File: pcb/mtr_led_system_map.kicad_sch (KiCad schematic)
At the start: 489 parts, among them J1 USB_C_Receptacle_USB2.0_16P, U1 ESP32-S3-WROOM-1, U2 AP2112K-3.3

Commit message: Updated the schematic to use dual red/yellow LEDs
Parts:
- removed DR_DOOR_1, DY_ISL_ADM1, DY_ISL_CAB1, DY_ISL_CEN1, DY_ISL_CHW1, DY_ISL_FOH1, DY_ISL_HAH1, DY_ISL_HFC1, DY_ISL_HKU1, DY_ISL_KET1, DY_ISL_NOP1, DY_ISL_POA1, DY_ISL_QUB1, DY_ISL_SHW1, DY_ISL_SKW1, DY_ISL_SWH1, DY_ISL_SYP1, DY_ISL_TAK1, DY_ISL_TIH1, DY_ISL_WAC1, DY_KTL_CHH1, DY_KTL_DIH1, DY_KTL_HOM1, DY_KTL_KOB1, DY_KTL_KOT1, DY_KTL_KWT1, DY_KTL_LAT1, DY_KTL_LOF1, DY_KTL_MOK1, DY_KTL_NTK1, DY_KTL_PRE1, DY_KTL_SKM1, DY_KTL_TIK1, DY_KTL_WHA1, DY_KTL_WTS1, DY_KTL_YAT1, DY_KTL_YMT1, DY_TKL_LHP1, DY_TKL_NOP1, DY_TKL_QUB1, DY_TKL_TIK1, DY_TKL_TKO1, DY_TKL_YAT1, DY_TWL_ADM1, DY_TWL_CEN1, DY_TWL_CSW1, DY_TWL_JOR1, DY_TWL_KWF1, DY_TWL_KWH1, DY_TWL_LAK1, DY_TWL_LCK1, DY_TWL_MEF1, DY_TWL_MOK1, DY_TWL_PRE1, DY_TWL_SSP1, DY_TWL_TST1, DY_TWL_TSW1, DY_TWL_TWH1, DY_TWL_YMT1: YELLOW, LED_SMD:LED_0805_2012Metric, symbol Device:LED
- removed DR_DOOR_2: GREEN, LED_SMD:LED_0805_2012Metric, symbol Device:LED
- removed DR_ISL_ADM1, DR_ISL_CAB1, DR_ISL_CEN1, DR_ISL_CHW1, DR_ISL_FOH1, DR_ISL_HFC1, DR_ISL_HKU1, DR_ISL_KET1, DR_ISL_NOP1, DR_ISL_QUB1, DR_ISL_SHW1, DR_ISL_SKW1, DR_ISL_SWH1, DR_ISL_SYP1, DR_ISL_TAK1, DR_ISL_TIH1, DR_ISL_WAC1, DR_KTL_CHH1, DR_KTL_DIH1, DR_KTL_HOM1, DR_KTL_KOB1, DR_KTL_KOT1, DR_KTL_KWT1, DR_KTL_LAT1, DR_KTL_LOF1, DR_KTL_MOK1, DR_KTL_NTK1, DR_KTL_PRE1, DR_KTL_SKM1, DR_KTL_TIK1, DR_KTL_WHA1, DR_KTL_WTS1, DR_KTL_YAT1, DR_KTL_YMT1, DR_TKL_HAH1, DR_TKL_LHP1, DR_TKL_NOP1, DR_TKL_POA1, DR_TKL_QUB1, DR_TKL_TIK1, DR_TKL_TKO1, DR_TKL_YAT1, DR_TWL_ADM1, DR_TWL_CEN1, DR_TWL_CSW1, DR_TWL_JOR1, DR_TWL_KWF1, DR_TWL_KWH1, DR_TWL_LAK1, DR_TWL_LCK1, DR_TWL_MEF1, DR_TWL_MOK1, DR_TWL_PRE1, DR_TWL_SSP1, DR_TWL_TST1, DR_TWL_TSW1, DR_TWL_TWH1, DR_TWL_YMT1: RED, LED_SMD:LED_0805_2012Metric, symbol Device:LED
- removed R1, R109, R110, R111, R112, R113, R114, R115, R116, R133, R134, R135, R136, R137, R138, R139, R140, R155, R156, R157, R158, R159, R160, R169, R170, R171, R172, R181, R182, R183, R184, R185, R186, R187, R188, R189, R190, R191, R192, R193, R194, R195, R196, R197, R198, R199, R2, R200, R201, R202, R203, R204, R205, R206, R207, R208, R209, R210, R211, R212, R213, R214, R215, R216, R217, R218, R219, R220, R221, R222, R223, R224, R225, R226, R227, R228, R229, R230, R231, R232, R233, R234, R235, R236, R237, R238, R27, R28, R29, R3, R30, R31, R32, R33, R34, R4, R5, R53, R54, R55, R56, R57, R58, R59, R6, R60, R7, R8, R83, R84, R85, R86, R87, R88, R89, R90: 220R, Resistor_SMD:R_0603_1608Metric, symbol Device:R
- added D_DOOR_G1: GREEN, LED_SMD:LED_0805_2012Metric, symbol Device:LED
- added D_DOOR_Y1: YELLOW, LED_SMD:LED_0805_2012Metric, symbol Device:LED
- added D_ISL_ADM1, D_ISL_CEN1, D_ISL_CHW1, D_ISL_CWB1, D_ISL_FOH1, D_ISL_HFC1, D_ISL_HKU1, D_ISL_KET1, D_ISL_NOP1, D_ISL_QUB1, D_ISL_SHW1, D_ISL_SKW1, D_ISL_SWH1, D_ISL_SYP1, D_ISL_TAK1, D_ISL_TIH1, D_ISL_WAC1, D_KTL_CHH1, D_KTL_DIH1, D_KTL_HOM1, D_KTL_KOB1, D_KTL_KOT1, D_KTL_KWT1, D_KTL_LAT1, D_KTL_LOF1, D_KTL_MOK1, D_KTL_NTK1, D_KTL_PRE1, D_KTL_SKM1, D_KTL_TIK1, D_KTL_WHA1, D_KTL_WTS1, D_KTL_YAT1, D_KTL_YMT1, D_TKL_HAH1, D_TKL_LHP1, D_TKL_NOP1, D_TKL_POA1, D_TKL_QUB1, D_TKL_TIK1, D_TKL_TKO1, D_TKL_YAT1, D_TWL_ADM1, D_TWL_CEN1, D_TWL_CSW1, D_TWL_JOR1, D_TWL_KWF1, D_TWL_KWH1, D_TWL_LAK1, D_TWL_LCK1, D_TWL_MEF1, D_TWL_MOK1, D_TWL_PRE1, D_TWL_SSP1, D_TWL_TST1, D_TWL_TSW1, D_TWL_TWH1, D_TWL_YMT1: RED_YELLOW, LED_SMD:LED_Kingbright_APHBM2012_2x1.25mm, symbol Device:LED_Dual_AKKA
- added R647, R648, R649, R650, R667, R668, R669, R670, R671, R672, R673, R674, R675, R676, R677, R678, R695, R696, R697, R698, R699, R700, R701, R702, R703, R704, R705, R706, R707, R708, R709, R710, R727, R728, R729, R730, R731, R732, R733, R734, R735, R736, R737, R738, R739, R740, R741, R742, R759, R760, R761, R762, R763, R764, R765, R766, R767, R768, R769, R770, R771, R772, R773, R774, R791, R792, R793, R794, R795, R796, R797, R798, R799, R800, R801, R802, R803, R804, R805, R806, R823, R824, R825, R826, R827, R828, R829, R830, R831, R832, R833, R834, R835, R836, R837, R838, R855, R856, R857, R858, R859, R860, R861, R862, R863, R864, R865, R866, R867, R868, R869, R870, R887, R888, R895, R896: 220R, Resistor_SMD:R_0603_1608Metric, symbol Device:R
- renumbered DG_ISL_ADM_CEN1 to D_ISL_ADM_CEN1, DG_ISL_ADM_WAC1 to D_ISL_ADM_WAC1, DG_ISL_CAB_TIH1 to D_ISL_CAB_TIH1, DG_ISL_CAB_WAC1 to D_ISL_CAB_WAC1, DG_ISL_CEN_ADM1 to D_ISL_CEN_ADM1, DG_ISL_CEN_SHW1 to D_ISL_CEN_SHW1, DG_ISL_CHW_HFC1 to D_ISL_CHW_HFC1, DG_ISL_FOH_NOP1 to D_ISL_FOH_NOP1, DG_ISL_FOH_TIH1 to D_ISL_FOH_TIH1, DG_ISL_HFC_CHW1 to D_ISL_HFC_CHW1, DG_ISL_HFC_SKW1 to D_ISL_HFC_SKW1, DG_ISL_HKU_KET1 to D_ISL_HKU_KET1, DG_ISL_HKU_SYP1 to D_ISL_HKU_SYP1, DG_ISL_KET_HKU1 to D_ISL_KET_HKU1, DG_ISL_NOP_FOH1 to D_ISL_NOP_FOH1, DG_ISL_NOP_QUB1 to D_ISL_NOP_QUB1, DG_ISL_QUB_NOP1 to D_ISL_QUB_NOP1, DG_ISL_QUB_TAK1 to D_ISL_QUB_TAK1, DG_ISL_SHW_CEN1 to D_ISL_SHW_CEN1, DG_ISL_SHW_SYP1 to D_ISL_SHW_SYP1, DG_ISL_SKW_HFC1 to D_ISL_SKW_HFC1, DG_ISL_SKW_SWH1 to D_ISL_SKW_SWH1, DG_ISL_SWH_SKW1 to D_ISL_SWH_SKW1, DG_ISL_SWH_TAK1 to D_ISL_SWH_TAK1, DG_ISL_SYP_HKU1 to D_ISL_SYP_HKU1, DG_ISL_SYP_SHW1 to D_ISL_SYP_SHW1, DG_ISL_TAK_QUB1 to D_ISL_TAK_QUB1, DG_ISL_TAK_SWH1 to D_ISL_TAK_SWH1, DG_ISL_TIH_CAB1 to D_ISL_TIH_CAB1, DG_ISL_TIH_FOH1 to D_ISL_TIH_FOH1, DG_ISL_WAC_ADM1 to D_ISL_WAC_ADM1, DG_ISL_WAC_CAB1 to D_ISL_WAC_CAB1, DG_KTL_CHH_DIH1 to D_KTL_CHH_DIH1, DG_KTL_CHH_KOB1 to D_KTL_CHH_KOB1, DG_KTL_DIH_CHH1 to D_KTL_DIH_CHH1, DG_KTL_DIH_WTS1 to D_KTL_DIH_WTS1, DG_KTL_HOM_WHA1 to D_KTL_HOM_WHA1, DG_KTL_HOM_YMT1 to D_KTL_HOM_YMT1, DG_KTL_KOB_CHH1 to D_KTL_KOB_CHH1, DG_KTL_KOB_NTK1 to D_KTL_KOB_NTK1, DG_KTL_KOT_LOF1 to D_KTL_KOT_LOF1, DG_KTL_KOT_SKM1 to D_KTL_KOT_SKM1, DG_KTL_KWT_LAT1 to D_KTL_KWT_LAT1, DG_KTL_KWT_NTK1 to D_KTL_KWT_NTK1, DG_KTL_LAT_KWT1 to D_KTL_LAT_KWT1, DG_KTL_LAT_YAT1 to D_KTL_LAT_YAT1, DG_KTL_LOF_KOT1 to D_KTL_LOF_KOT1, DG_KTL_LOF_WTS1 to D_KTL_LOF_WTS1, DG_KTL_MOK_PRE1 to D_KTL_MOK_PRE1, DG_KTL_MOK_YMT1 to D_KTL_MOK_YMT1, DG_KTL_NTK_KOB1 to D_KTL_NTK_KOB1, DG_KTL_NTK_KWT1 to D_KTL_NTK_KWT1, DG_KTL_PRE_MOK1 to D_KTL_PRE_MOK1, DG_KTL_PRE_SKM1 to D_KTL_PRE_SKM1, DG_KTL_SKM_KOT1 to D_KTL_SKM_KOT1, DG_KTL_SKM_PRE1 to D_KTL_SKM_PRE1, DG_KTL_TIK_YAT1 to D_KTL_TIK_YAT1, DG_KTL_WHA_HOM1 to D_KTL_WHA_HOM1, DG_KTL_WTS_DIH1 to D_KTL_WTS_DIH1, DG_KTL_WTS_LOF1 to D_KTL_WTS_LOF1, DG_KTL_YAT_LAT1 to D_KTL_YAT_LAT1, DG_KTL_YAT_TIK1 to D_KTL_YAT_TIK1, DG_KTL_YMT_HOM1 to D_KTL_YMT_HOM1, DG_KTL_YMT_MOK1 to D_KTL_YMT_MOK1, DY_TCL_HOK1 to D_TCL_HOK1, DY_TCL_KOW1 to D_TCL_KOW1, DY_TCL_LAK1 to D_TCL_LAK1, DY_TCL_NAC1 to D_TCL_NAC1, DY_TCL_OLY1 to D_TCL_OLY1, DY_TCL_SUN1 to D_TCL_SUN1, DY_TCL_TSY1 to D_TCL_TSY1, DY_TCL_TUC1 to D_TCL_TUC1, DG_TKL_HAH_POA1 to D_TKL_HAH_POA1, DG_TKL_HAH_TKO1 to D_TKL_HAH_TKO1, DG_TKL_LHP_TKO1 to D_TKL_LHP_TKO1, DG_TKL_NOP_QUB1 to D_TKL_NOP_QUB1, DG_TKL_POA_HAH1 to D_TKL_POA_HAH1, DG_TKL_QUB_NOP1 to D_TKL_QUB_NOP1, DG_TKL_QUB_YAT1 to D_TKL_QUB_YAT1, DG_TKL_TIK_TKO1 to D_TKL_TIK_TKO1, DG_TKL_TIK_YAT1 to D_TKL_TIK_YAT1, DG_TKL_TKO_HAH1 to D_TKL_TKO_HAH1, DG_TKL_TKO_LHP1 to D_TKL_TKO_LHP1, DG_TKL_TKO_TIK1 to D_TKL_TKO_TIK1, DG_TKL_YAT_QUB1 to D_TKL_YAT_QUB1, DG_TKL_YAT_TIK1 to D_TKL_YAT_TIK1, DG_TWL_ADM_CEN1 to D_TWL_ADM_CEN1, DG_TWL_ADM_TST1 to D_TWL_ADM_TST1, DG_TWL_CEN_ADM1 to D_TWL_CEN_ADM1, DG_TWL_CSW_LCK1 to D_TWL_CSW_LCK1, DG_TWL_CSW_SSP1 to D_TWL_CSW_SSP1, DG_TWL_JOR_TST1 to D_TWL_JOR_TST1, DG_TWL_JOR_YMT1 to D_TWL_JOR_YMT1, DG_TWL_KWF_KWH1 to D_TWL_KWF_KWH1, DG_TWL_KWF_LAK1 to D_TWL_KWF_LAK1, DG_TWL_KWH_KWF1 to D_TWL_KWH_KWF1, DG_TWL_KWH_TWH1 to D_TWL_KWH_TWH1, DG_TWL_LAK_KWF1 to D_TWL_LAK_KWF1, DG_TWL_LAK_MEF1 to D_TWL_LAK_MEF1, DG_TWL_LCK_CSW1 to D_TWL_LCK_CSW1, DG_TWL_LCK_MEF1 to D_TWL_LCK_MEF1, DG_TWL_MEF_LAK1 to D_TWL_MEF_LAK1, DG_TWL_MEF_LCK1 to D_TWL_MEF_LCK1, DG_TWL_MOK_PRE1 to D_TWL_MOK_PRE1, DG_TWL_MOK_YMT1 to D_TWL_MOK_YMT1, DG_TWL_PRE_MOK1 to D_TWL_PRE_MOK1, DG_TWL_PRE_SSP1 to D_TWL_PRE_SSP1, DG_TWL_SSP_CSW1 to D_TWL_SSP_CSW1, DG_TWL_SSP_PRE1 to D_TWL_SSP_PRE1, DG_TWL_TST_ADM1 to D_TWL_TST_ADM1, DG_TWL_TST_JOR1 to D_TWL_TST_JOR1, DG_TWL_TSW_TWH1 to D_TWL_TSW_TWH1, DG_TWL_TWH_KWH1 to D_TWL_TWH_KWH1, DG_TWL_TWH_TSW1 to D_TWL_TWH_TSW1, DG_TWL_YMT_JOR1 to D_TWL_YMT_JOR1, DG_TWL_YMT_MOK1 to D_TWL_YMT_MOK1
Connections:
- net +5V: now also D_DOOR_G1.2 (A), D_DOOR_Y1.2 (A), D_ISL_ADM1.1 (A1), D_ISL_ADM1.4 (A2), D_ISL_CEN1.1 (A1), D_ISL_CEN1.4 (A2), D_ISL_CHW1.1 (A1), D_ISL_CHW1.4 (A2), D_ISL_CWB1.1 (A1), D_ISL_CWB1.4 (A2), D_ISL_FOH1.1 (A1), D_ISL_FOH1.4 (A2), D_ISL_HFC1.1 (A1), D_ISL_HFC1.4 (A2), D_ISL_HKU1.1 (A1), D_ISL_HKU1.4 (A2), D_ISL_KET1.1 (A1), D_ISL_KET1.4 (A2), D_ISL_NOP1.1 (A1), D_ISL_NOP1.4 (A2), D_ISL_QUB1.1 (A1), D_ISL_QUB1.4 (A2), D_ISL_SHW1.1 (A1), D_ISL_SHW1.4 (A2), D_ISL_SKW1.1 (A1), D_ISL_SKW1.4 (A2), D_ISL_SWH1.1 (A1), D_ISL_SWH1.4 (A2), D_ISL_SYP1.1 (A1), D_ISL_SYP1.4 (A2), D_ISL_TAK1.1 (A1), D_ISL_TAK1.4 (A2), D_ISL_TIH1.1 (A1), D_ISL_TIH1.4 (A2), D_ISL_WAC1.1 (A1), D_ISL_WAC1.4 (A2), D_KTL_CHH1.1 (A1), D_KTL_CHH1.4 (A2), D_KTL_DIH1.1 (A1), D_KTL_DIH1.4 (A2), D_KTL_HOM1.1 (A1), D_KTL_HOM1.4 (A2), D_KTL_KOB1.1 (A1), D_KTL_KOB1.4 (A2), D_KTL_KOT1.1 (A1), D_KTL_KOT1.4 (A2), D_KTL_KWT1.1 (A1), D_KTL_KWT1.4 (A2), D_KTL_LAT1.1 (A1), D_KTL_LAT1.4 (A2), D_KTL_LOF1.1 (A1), D_KTL_LOF1.4 (A2), D_KTL_MOK1.1 (A1), D_KTL_MOK1.4 (A2), D_KTL_NTK1.1 (A1), D_KTL_NTK1.4 (A2), D_KTL_PRE1.1 (A1), D_KTL_PRE1.4 (A2), D_KTL_SKM1.1 (A1), D_KTL_SKM1.4 (A2), D_KTL_TIK1.1 (A1), D_KTL_TIK1.4 (A2), D_KTL_WHA1.1 (A1), D_KTL_WHA1.4 (A2), D_KTL_WTS1.1 (A1), D_KTL_WTS1.4 (A2), D_KTL_YAT1.1 (A1), D_KTL_YAT1.4 (A2), D_KTL_YMT1.1 (A1), D_KTL_YMT1.4 (A2), D_TKL_HAH1.1 (A1), D_TKL_HAH1.4 (A2), D_TKL_LHP1.1 (A1), D_TKL_LHP1.4 (A2), D_TKL_NOP1.1 (A1), D_TKL_NOP1.4 (A2), D_TKL_POA1.1 (A1), D_TKL_POA1.4 (A2), D_TKL_QUB1.1 (A1), D_TKL_QUB1.4 (A2), D_TKL_TIK1.1 (A1), D_TKL_TIK1.4 (A2), D_TKL_TKO1.1 (A1), D_TKL_TKO1.4 (A2), D_TKL_YAT1.1 (A1), D_TKL_YAT1.4 (A2), D_TWL_ADM1.1 (A1), D_TWL_ADM1.4 (A2), D_TWL_CEN1.1 (A1), D_TWL_CEN1.4 (A2), D_TWL_CSW1.1 (A1), D_TWL_CSW1.4 (A2), D_TWL_JOR1.1 (A1), D_TWL_JOR1.4 (A2), D_TWL_KWF1.1 (A1), D_TWL_KWF1.4 (A2), D_TWL_KWH1.1 (A1), D_TWL_KWH1.4 (A2), D_TWL_LAK1.1 (A1), D_TWL_LAK1.4 (A2), D_TWL_LCK1.1 (A1), D_TWL_LCK1.4 (A2), D_TWL_MEF1.1 (A1), D_TWL_MEF1.4 (A2), D_TWL_MOK1.1 (A1), D_TWL_MOK1.4 (A2), D_TWL_PRE1.1 (A1), D_TWL_PRE1.4 (A2), D_TWL_SSP1.1 (A1), D_TWL_SSP1.4 (A2), D_TWL_TST1.1 (A1), D_TWL_TST1.4 (A2), D_TWL_TSW1.1 (A1), D_TWL_TSW1.4 (A2), D_TWL_TWH1.1 (A1), D_TWL_TWH1.4 (A2), D_TWL_YMT1.1 (A1), D_TWL_YMT1.4 (A2)
- net at R154.2: now also D_DOOR_G1.1 (K)
- net at R153.2: now also D_DOOR_Y1.1 (K)
- net ISL R3 + TKL R1/LED_1 renamed R8/LED_3
- net ISL R3 + TKL R1/LED_2 renamed R8/LED_4
- net TCL Y/LED_1 renamed TCL_Y1
- new net: D_KTL_PRE1.2 (K1), R699.2
- new net: D_TWL_MEF1.3 (K2), R741.2
- new net: D_ISL_QUB1.2 (K1), R797.2
- new net: D_TWL_TSW1.2 (K1), R728.2
- new net: D_KTL_DIH1.2 (K1), R677.2
- new net: D_KTL_NTK1.3 (K2), R672.2
- new net: D_TWL_LCK1.2 (K1), R734.2
- new net: D_KTL_HOM1.2 (K1), R702.2
- new net: D_TWL_JOR1.2 (K1), R764.2
- new net: D_TKL_LHP1.3 (K2), R867.2
- new net: D_ISL_CWB1.2 (K1), R825.2
- new net: D_ISL_HFC1.2 (K1), R793.2
- new net: D_TKL_YAT1.2 (K1), R862.2
- new net: D_ISL_SKW1.3 (K2), R802.2
- new net: D_KTL_MOK1.2 (K1), R700.2
- new net: D_TWL_TST1.3 (K2), R773.2
- new net: D_ISL_SHW1.2 (K1), R829.2
- new net: D_KTL_KOT1.2 (K1), R697.2
- new net: D_ISL_HKU1.2 (K1), R855.2
- new net: D_TWL_PRE1.3 (K2), R769.2
- new net: D_TKL_HAH1.3 (K2), R866.2
- new net: D_ISL_SYP1.2 (K1), R830.2
- new net: D_ISL_SYP1.3 (K2), R838.2
- new net: D_TKL_NOP1.2 (K1), R888.2
- new net: D_ISL_QUB1.3 (K2), R805.2
- new net: D_TWL_TSW1.3 (K2), R736.2
- new net: D_TWL_CEN1.3 (K2), R799.2
- new net: D_KTL_LOF1.3 (K2), R704.2
- new net: D_TWL_PRE1.2 (K1), R761.2
- new net: D_TWL_MEF1.2 (K1), R733.2
- new net: D_KTL_TIK1.3 (K2), R648.2
- new net: D_KTL_YAT1.2 (K1), R649.2
- new net: D_TWL_SSP1.2 (K1), R760.2
- new net: D_TWL_SSP1.3 (K2), R768.2
- new net: D_KTL_HOM1.3 (K2), R710.2
- new net: D_KTL_MOK1.3 (K2), R708.2
- new net: D_KTL_YAT1.3 (K2), R650.2
- new net: D_TWL_TST1.2 (K1), R765.2
- new net: D_TWL_JOR1.3 (K2), R772.2
- new net: D_TWL_LCK1.3 (K2), R742.2
- new net: D_TWL_TWH1.2 (K1), R729.2
- new net: D_KTL_LOF1.2 (K1), R696.2
- new net: D_TWL_TWH1.3 (K2), R737.2
- new net: D_KTL_CHH1.2 (K1), R675.2
- new net: D_KTL_CHH1.3 (K2), R676.2
- new net: D_ISL_NOP1.2 (K1), R798.2
- new net: D_KTL_PRE1.3 (K2), R707.2
- new net: D_ISL_SWH1.2 (K1), R795.2
- new net: D_KTL_WTS1.2 (K1), R695.2
- new net: D_KTL_WTS1.3 (K2), R703.2
- new net: D_ISL_SHW1.3 (K2), R837.2
- new net: D_TWL_ADM1.2 (K1), R766.2
- new net: D_TWL_ADM1.3 (K2), R774.2
- new net: D_KTL_SKM1.2 (K1), R698.2
- new net: D_KTL_SKM1.3 (K2), R706.2
- new net: D_ISL_KET1.3 (K2), R864.2
- new net: D_ISL_TAK1.2 (K1), R796.2
- new net: D_ISL_ADM1.3 (K2), R835.2
- new net: D_KTL_WHA1.2 (K1), R727.2
- new net: D_KTL_WHA1.3 (K2), R735.2
- new net: D_ISL_WAC1.2 (K1), R826.2
- new net: D_ISL_CEN1.2 (K1), R828.2
- new net: D_ISL_CEN1.3 (K2), R836.2
- new net: D_ISL_ADM1.2 (K1), R827.2
- new net: D_ISL_KET1.2 (K1), R856.2
- new net: D_KTL_KOB1.2 (K1), R673.2
- new net: D_TKL_TIK1.3 (K2), R869.2
- new net: D_KTL_KOT1.3 (K2), R705.2
- new net: D_TWL_LAK1.2 (K1), R732.2
- new net: D_TWL_LAK1.3 (K2), R740.2
- new net: D_TWL_KWH1.3 (K2), R738.2
- new net: D_KTL_KWT1.3 (K2), R670.2
- new net: D_TKL_TKO1.3 (K2), R868.2
- new net: D_KTL_YMT1.2 (K1), R701.2
- new net: D_KTL_YMT1.3 (K2), R709.2
- new net: D_TKL_NOP1.3 (K2), R896.2
- new net: D_TWL_YMT1.2 (K1), R763.2
- new net: D_TWL_YMT1.3 (K2), R771.2
- new net: D_ISL_SWH1.3 (K2), R803.2
- new net: D_TKL_QUB1.3 (K2), R895.2
- new net: D_TWL_MOK1.2 (K1), R762.2
- new net: D_TKL_YAT1.3 (K2), R870.2
- new net: D_TWL_KWF1.3 (K2), R739.2
- new net: D_KTL_NTK1.2 (K1), R671.2
- new net: D_TWL_CSW1.2 (K1), R759.2
- new net: D_KTL_KWT1.2 (K1), R669.2
- new net: D_ISL_CHW1.2 (K1), R792.2
- new net: D_ISL_CHW1.3 (K2), R800.2
- new net: D_TKL_TIK1.2 (K1), R861.2
- new net: D_KTL_DIH1.3 (K2), R678.2
- new net: D_KTL_LAT1.2 (K1), R667.2
- new net: D_KTL_LAT1.3 (K2), R668.2
- new net: D_ISL_HFC1.3 (K2), R801.2
- new net: D_TWL_MOK1.3 (K2), R770.2
- new net: D_ISL_HKU1.3 (K2), R863.2
- new net: D_TWL_KWH1.2 (K1), R730.2
- new net: D_ISL_WAC1.3 (K2), R834.2
- new net: D_KTL_KOB1.3 (K2), R674.2
- new net: D_TKL_TKO1.2 (K1), R860.2
- new net: D_ISL_CWB1.3 (K2), R833.2
- new net: D_TKL_HAH1.2 (K1), R858.2
- new net: D_ISL_SKW1.2 (K1), R794.2
- new net: D_TKL_LHP1.2 (K1), R859.2
- new net: D_ISL_TAK1.3 (K2), R804.2
- new net: D_ISL_TIH1.2 (K1), R824.2
- new net: D_ISL_TIH1.3 (K2), R832.2
- new net: D_KTL_TIK1.2 (K1), R647.2
- new net: D_ISL_NOP1.3 (K2), R806.2
- new net: D_ISL_FOH1.2 (K1), R823.2
- new net: D_TWL_KWF1.2 (K1), R731.2
- new net: D_TWL_CSW1.3 (K2), R767.2
- new net: D_ISL_FOH1.3 (K2), R831.2
- new net: D_TWL_CEN1.2 (K1), R791.2
- new net: D_TKL_QUB1.2 (K1), R887.2
- new net: D_TKL_POA1.2 (K1), R857.2
- new net: D_TKL_POA1.3 (K2), R865.2
- new net ISL_Y1: R800.1, R801.1, R802.1, R803.1, R804.1, R805.1
- new net ISL_Y2: R806.1, R831.1, R832.1, R833.1, R834.1, R835.1
- new net ISL_Y3: R836.1, R837.1, R838.1, R863.1, R864.1
- new net KTL_Y1: R648.1
- new net KTL_Y2: R650.1, R668.1, R670.1, R672.1, R674.1, R676.1, R678.1, R703.1, R704.1, R705.1, R706.1, R707.1
- new net KTL_Y3: R708.1
- new net KTL_Y4: R709.1, R710.1, R735.1
- new net R1/LED_1: R647.1
- new net R1/LED_2: R649.1
- new net R1/LED_3: R667.1
- new net R1/LED_4: R669.1
- new net R1/LED_5: R671.1
- new net R1/LED_6: R673.1
- new net R1/LED_7: R675.1
- new net R1/LED_8: R677.1
- new net R2/LED_1: R695.1
- new net R2/LED_2: R696.1
- new net R2/LED_3: R697.1
- new net R2/LED_4: R698.1
- new net R2/LED_5: R699.1
- new net R2/LED_6: R700.1
- new net R2/LED_7: R701.1
- new net R2/LED_8: R702.1
- new net R3/LED_1: R727.1
- new net R3/LED_2: R728.1
- new net R3/LED_3: R729.1
- new net R3/LED_4: R730.1
- new net R3/LED_5: R731.1
- new net R3/LED_6: R732.1
- new net R3/LED_7: R733.1
- new net R3/LED_8: R734.1
- new net R4/LED_1: R759.1
- new net R4/LED_2: R760.1
- new net R4/LED_3: R761.1
- new net R4/LED_4: R762.1
- new net R4/LED_5: R763.1
- new net R4/LED_6: R764.1
- new net R4/LED_7: R765.1
- new net R4/LED_8: R766.1
- new net R5/LED_1: R791.1
- new net R5/LED_2: R792.1
- new net R5/LED_3: R793.1
- new net R5/LED_4: R794.1
- new net R5/LED_5: R795.1
- new net R5/LED_6: R796.1
- new net R5/LED_7: R797.1
- new net R5/LED_8: R798.1
- new net R6/LED_1: R823.1
- new net R6/LED_2: R824.1
- new net R6/LED_3: R825.1
- new net R6/LED_4: R826.1
- new net R6/LED_5: R827.1
- new net R6/LED_6: R828.1
- new net R6/LED_7: R829.1
- new net R6/LED_8: R830.1
- new net R7/LED_1: R855.1
- new net R7/LED_2: R856.1
- new net R7/LED_3: R857.1
- new net R7/LED_4: R858.1
- new net R7/LED_5: R859.1
- new net R7/LED_6: R860.1
- new net R7/LED_7: R861.1
- new net R7/LED_8: R862.1
- new net R8/LED_1: R887.1
- new net R8/LED_2: R888.1
- new net TKL_Y1: R865.1, R866.1
- new net TKL_Y2: R867.1
- new net TKL_Y3: R868.1, R869.1
- new net TKL_Y4: R870.1, R895.1
- new net TKL_Y5: R896.1
- new net TWL_Y1: R736.1, R737.1, R738.1, R739.1, R740.1, R741.1, R742.1, R767.1, R768.1, R769.1
- new net TWL_Y2: R770.1
- new net TWL_Y3: R771.1, R772.1, R773.1, R774.1
- new net TWL_Y4: R799.1
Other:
- sheet ISL G2 renamed G9
- sheet ISL G3 renamed G10
- sheet ISL G4 renamed G11
- sheet ISL G5 + TKL G1 renamed G12
- sheet KTL G1 renamed G1
- sheet KTL G2 renamed G2
- sheet KTL G3 renamed G3
- sheet KTL G4 renamed G4
- sheet TKL G2 renamed G13
- sheet TKL G3 renamed G14
- sheet TWL G1 renamed G5
- sheet TWL G2 renamed G6
- sheet TWL G3 renamed G7
- sheet TWL G4 + ISL G1 renamed G8
- removed sheet ISL R2
- removed sheet ISL R3 + TKL R1
- removed sheet ISL Y + TKL Y
- removed sheet KTL R1
- removed sheet KTL R2
- removed sheet KTL R3 + TWL R1
- removed sheet KTL Y + TWL Y
- removed sheet TCL Y
- removed sheet TKL R2 + KTL Y1
- removed sheet TWL R2
- removed sheet TWL R3 + ISL R1
- added sheet R1 (led_group_595.kicad_sch)
- added sheet R2 (led_group_595.kicad_sch)
- added sheet R3 (led_group_595.kicad_sch)
- added sheet R4 (led_group_595.kicad_sch)
- added sheet R5 (led_group_595.kicad_sch)
- added sheet R6 (led_group_595.kicad_sch)
- added sheet R7 (led_group_595.kicad_sch)
- added sheet R8 (led_group_595.kicad_sch)
- added sheet Y1 (led_group_595.kicad_sch)
- added sheet Y2 (led_group_595.kicad_sch)
- added sheet Y3 (led_group_595.kicad_sch)
- moved on the sheet: C1, C2, C3, C4, C5, C6, D_ISL_ADM_CEN1, D_ISL_ADM_WAC1, D_ISL_CAB_TIH1, D_ISL_CAB_WAC1, D_ISL_CEN_ADM1, D_ISL_CEN_SHW1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

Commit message: Circuit rewrite to put LEDs closer together for the shift registers
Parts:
- removed R153, R154: 220R, Resistor_SMD:R_0603_1608Metric, symbol Device:R
- added R205, R206: 220R, Resistor_SMD:R_0603_1608Metric, symbol Device:R
- renumbered R728 to R1, R117 to R10, R768 to R100, R161 to R101, R162 to R102, R769 to R103, R163 to R104, R164 to R105, R47 to R106, R48 to R107, R832 to R108, R49 to R109, R118 to R11, R50 to R110, R833 to R111, R69 to R112, R70 to R113, R710 to R114, R97 to R115, R98 to R116, R735 to R117, R151 to R118, R152 to R119, R737 to R12, R896 to R120, R762 to R121, R763 to R122, R764 to R123, R826 to R124, R827 to R125, R828 to R126, R857 to R127, R858 to R128, R859 to R129, R119 to R13, R770 to R130, R165 to R131, R166 to R132, R771 to R133, R167 to R134, R168 to R135, R772 to R136, R834 to R137, R71 to R138, R72 to R139, R120 to R14, R835 to R140, R73 to R141, R74 to R142, R836 to R143, R865 to R144, R105 to R145, R106 to R146, R866 to R147, R125 to R148, R126 to R149, R738 to R15, R867 to R150, R765 to R151, R766 to R152, R647 to R153, R649 to R154, R667 to R155, R860 to R156, R861 to R157, R173 to R158, R174 to R159, R800 to R16, R773 to R160, R175 to R161, R176 to R162, R774 to R163, R177 to R164, R178 to R165, R648 to R166, R9 to R167, R10 to R168, R650 to R169, R179 to R17, R11 to R170, R12 to R171, R668 to R172, R127 to R173, R128 to R174, R868 to R175, R129 to R176, R130 to R177, R869 to R178, R131 to R179, R180 to R18, R132 to R180, R791 to R181, R829 to R182, R669 to R183, R671 to R184, R862 to R185, R887 to R186, R799 to R187, R75 to R188, R76 to R189, R801 to R19, R837 to R190, R99 to R191, R100 to R192, R13 to R193, R14 to R194, R670 to R195, R15 to R196, R16 to R197, R672 to R198, R35 to R199, R729 to R2, R17 to R20, R36 to R200, R870 to R201, R149 to R202, R150 to R203, R895 to R204, R830 to R207, R855 to R208, R856 to R209, R18 to R21, R673 to R210, R675 to R211, R677 to R212, R838 to R213, R101 to R214, R102 to R215, R863 to R216, R103 to R217, R104 to R218, R864 to R219, R802 to R22, R674 to R220, R37 to R221, R38 to R222, R676 to R223, R39 to R224, R40 to R225, R678 to R226, R25 to R227, R26 to R228, R239 to R229, R41 to R23, R240 to R230, R241 to R231, R242 to R232, R243 to R233, R244 to R234, R245 to R235, R246 to R236, R51 to R237, R52 to R238, R77 to R239, R42 to R24, R78 to R240, R79 to R241, R80 to R242, R81 to R243, R82 to R244, R107 to R245, R108 to R246, R703 to R25, R61 to R26, R62 to R27, R704 to R28, R63 to R29, R730 to R3, R64 to R30, R731 to R31, R732 to R32, R795 to R33, R796 to R34, R697 to R35, R698 to R36, R699 to R37, R121 to R38, R122 to R39, R792 to R4, R739 to R40, R123 to R41, R124 to R42, R740 to R43, R141 to R44, R142 to R45, R19 to R46, R20 to R47, R803 to R48, R21 to R49, R793 to R5, R22 to R50, R804 to R51, R23 to R52, R24 to R53, R705 to R54, R65 to R55, R66 to R56, R706 to R57, R67 to R58, R68 to R59, R794 to R6, R707 to R60, R733 to R61, R734 to R62, R759 to R63, R797 to R64, R798 to R65, R823 to R66, R700 to R67, R701 to R68, R741 to R69, R695 to R7, R143 to R70, R144 to R71, R742 to R72, R145 to R73, R146 to R74, R767 to R75, R805 to R76, R43 to R77, R44 to R78, R806 to R79, R696 to R8, R45 to R80, R46 to R81, R831 to R82, R91 to R83, R92 to R84, R708 to R85, R93 to R86, R94 to R87, R709 to R88, R95 to R89, R736 to R9, R96 to R90, R760 to R91, R761 to R92, R824 to R93, R825 to R94, R702 to R95, R727 to R96, R888 to R97, R147 to R98, R148 to R99
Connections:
- net KTL_Y2: no longer R54.1, R57.1, R60.1
- net at D_DOOR_Y1.1 (K): now also R205.2
- net at D_DOOR_G1.1 (K): now also R206.2
- net DATA_G renamed DATA_3
- net DATA_R renamed DATA_1
- net DATA_Y renamed DATA_2
- net G1/LED_1 renamed S14/LED_3
- net G1/LED_2 renamed S14/LED_4
- net G1/LED_3 renamed S14/LED_6
- net G1/LED_4 renamed S14/LED_7
- net G1/LED_5 renamed S15/LED_1
- net G1/LED_6 renamed S15/LED_2
- net G1/LED_7 renamed S15/LED_4
- net G1/LED_8 renamed S15/LED_5
- net G10/LED_1 renamed S11/LED_3
- net G10/LED_2 renamed S11/LED_4
- net G10/LED_3 renamed S11/LED_6
- net G10/LED_4 renamed S11/LED_7
- net G10/LED_5 renamed S12/LED_1
- net G10/LED_6 renamed S12/LED_2
- net G10/LED_7 renamed S12/LED_4
- net G10/LED_8 renamed S12/LED_5
- net G11/LED_1 renamed S12/LED_7
- net G11/LED_2 renamed S12/LED_8
- net G11/LED_3 renamed S13/LED_3
- net G11/LED_4 renamed S13/LED_4
- net G11/LED_5 renamed S13/LED_6
- net G11/LED_6 renamed S13/LED_7
- net G11/LED_7 renamed S7/LED_4
- net G11/LED_8 renamed S7/LED_5
- net G12/LED_1 renamed S7/LED_7
- net G12/LED_2 renamed S7/LED_8
- net G12/LED_3 renamed S8/LED_3
- net G12/LED_4 renamed S8/LED_4
- net G12/LED_5 renamed S8/LED_6
- net G12/LED_6 renamed S8/LED_7
- net G12/LED_7 renamed S21/LED_3
- net G12/LED_8 renamed S21/LED_4
- net G13/LED_1 renamed S21/LED_6
- net G13/LED_2 renamed S21/LED_7
- net G13/LED_3 renamed S22/LED_1
- net G13/LED_4 renamed S22/LED_2
- net G13/LED_5 renamed S22/LED_4
- net G13/LED_6 renamed S22/LED_5
- net G13/LED_7 renamed S22/LED_7
- net G13/LED_8 renamed S22/LED_8
- net G14/LED_1 renamed S23/LED_3
- net G14/LED_2 renamed S23/LED_4
- net G14/LED_3 renamed S20/LED_6
- net G14/LED_4 renamed S20/LED_7
- net G2/LED_1 renamed S15/LED_7
- net G2/LED_2 renamed S15/LED_8
- net G2/LED_3 renamed S16/LED_3
- net G2/LED_4 renamed S16/LED_4
- net G2/LED_5 renamed S16/LED_6
- net G2/LED_6 renamed S16/LED_7
- net G2/LED_7 renamed S17/LED_1
- net G2/LED_8 renamed S17/LED_2
- net G3/LED_1 renamed S17/LED_4
- net G3/LED_2 renamed S17/LED_5
- net G3/LED_3 renamed S17/LED_7
- net G3/LED_4 renamed S17/LED_8
- net G3/LED_5 renamed S18/LED_3
- net G3/LED_6 renamed S18/LED_4
- net G3/LED_7 renamed S18/LED_6
- net G3/LED_8 renamed S18/LED_7
- net G4/LED_1 renamed S19/LED_1
- net G4/LED_2 renamed S19/LED_2
- net G4/LED_3 renamed S19/LED_4
- net G4/LED_4 renamed S19/LED_5
- net G4/LED_5 renamed S19/LED_7
- net G4/LED_6 renamed S19/LED_8
- net G4/LED_7 renamed S20/LED_3
- net G4/LED_8 renamed S20/LED_4
- net G5/LED_1 renamed S1/LED_3
- net G5/LED_2 renamed S1/LED_4
- net G5/LED_3 renamed S1/LED_6
- net G5/LED_4 renamed S1/LED_7
- net G5/LED_5 renamed S2/LED_1
- net G5/LED_6 renamed S2/LED_2
- net G5/LED_7 renamed S2/LED_4
- net G5/LED_8 renamed S2/LED_5
- net G6/LED_1 renamed S2/LED_7
- net G6/LED_2 renamed S2/LED_8
- net G6/LED_3 renamed S3/LED_3
- net G6/LED_4 renamed S3/LED_4
- net G6/LED_5 renamed S3/LED_6
- net G6/LED_6 renamed S3/LED_7
- net G6/LED_7 renamed S4/LED_1
- net G6/LED_8 renamed S4/LED_2
- net G7/LED_1 renamed S4/LED_4
- net G7/LED_2 renamed S4/LED_5
- net G7/LED_3 renamed S4/LED_7
- net G7/LED_4 renamed S4/LED_8
- net G7/LED_5 renamed S5/LED_3
- net G7/LED_6 renamed S5/LED_4
- net G7/LED_7 renamed S5/LED_6
- net G7/LED_8 renamed S5/LED_7
- net G8/LED_1 renamed S6/LED_1
- net G8/LED_2 renamed S6/LED_2
- net G8/LED_3 renamed S6/LED_4
- net G8/LED_4 renamed S6/LED_5
- net G8/LED_5 renamed S6/LED_7
- net G8/LED_6 renamed S6/LED_8
- net G8/LED_7 renamed S9/LED_3
- net G8/LED_8 renamed S9/LED_4
- net G9/LED_1 renamed S9/LED_6
- net G9/LED_2 renamed S9/LED_7
- net G9/LED_3 renamed S10/LED_1
- net G9/LED_4 renamed S10/LED_2
- net G9/LED_5 renamed S10/LED_4
- net G9/LED_6 renamed S10/LED_5
- net G9/LED_7 renamed S10/LED_7
- net G9/LED_8 renamed S10/LED_8
- net R1/LED_1 renamed S14/LED_2
- net R1/LED_2 renamed S14/LED_5
- net R1/LED_3 renamed S14/LED_8
- net R1/LED_4 renamed S15/LED_3
- net R1/LED_5 renamed S15/LED_6
- net R1/LED_6 renamed S16/LED_2
- net R1/LED_7 renamed S16/LED_5
- net R1/LED_8 renamed S16/LED_8
- net R2/LED_1 renamed S17/LED_3
- net R2/LED_2 renamed S17/LED_6
- net R2/LED_3 renamed S18/LED_2
- net R2/LED_4 renamed S18/LED_5
- net R2/LED_5 renamed S18/LED_8
- net R2/LED_6 renamed S19/LED_3
- net R2/LED_7 renamed S19/LED_6
- net R2/LED_8 renamed S20/LED_2
- net R3/LED_1 renamed S20/LED_5
- net R3/LED_2 renamed S1/LED_2
- net R3/LED_3 renamed S1/LED_5
- net R3/LED_4 renamed S1/LED_8
- net R3/LED_5 renamed S2/LED_3
- net R3/LED_6 renamed S2/LED_6
- net R3/LED_7 renamed S3/LED_2
- net R3/LED_8 renamed S3/LED_5
- net R4/LED_1 renamed S3/LED_8
- net R4/LED_2 renamed S4/LED_3
- net R4/LED_3 renamed S4/LED_6
- net R4/LED_4 renamed S5/LED_2
- net R4/LED_5 renamed S5/LED_5
- net R4/LED_6 renamed S5/LED_8
- net R4/LED_7 renamed S6/LED_3
- net R4/LED_8 renamed S6/LED_6
- net R5/LED_1 renamed S7/LED_2
- net R5/LED_2 renamed S9/LED_2
- net R5/LED_3 renamed S9/LED_5
- net R5/LED_4 renamed S9/LED_8
- net R5/LED_5 renamed S10/LED_3
- net R5/LED_6 renamed S10/LED_6
- net R5/LED_7 renamed S11/LED_2
- net R5/LED_8 renamed S11/LED_5
- net R6/LED_1 renamed S11/LED_8
- net R6/LED_2 renamed S12/LED_3
- net R6/LED_3 renamed S12/LED_6
- net R6/LED_4 renamed S13/LED_2
- net R6/LED_5 renamed S13/LED_5
- net R6/LED_6 renamed S13/LED_8
- net R6/LED_7 renamed S7/LED_6
- net R6/LED_8 renamed S8/LED_2
- net R7/LED_1 renamed S8/LED_5
- net R7/LED_2 renamed S8/LED_8
- net R7/LED_3 renamed S21/LED_2
- net R7/LED_4 renamed S21/LED_5
- net R7/LED_5 renamed S21/LED_8
- net R7/LED_6 renamed S22/LED_3
- net R7/LED_7 renamed S22/LED_6
- net R7/LED_8 renamed S23/LED_2
- net R8/LED_1 renamed S23/LED_5
- net R8/LED_2 renamed S20/LED_8
- net TWL_Y4 renamed S7/LED_3
- new net: R54.1, R57.1, R60.1
- new net S24/LED_1: R205.1
- new net S24/LED_2: R206.1
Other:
- removed sheet G1
- removed sheet G10
- removed sheet G11
- removed sheet G12
- removed sheet G13
- removed sheet G14
- removed sheet G2
- removed sheet G3
- removed sheet G4
- removed sheet G5
- removed sheet G6
- removed sheet G7
- removed sheet G8
- removed sheet G9
- removed sheet R1
- removed sheet R2
- removed sheet R3
- removed sheet R4
- removed sheet R5
- removed sheet R6
- removed sheet R7
- removed sheet R8
- removed sheet Y1
- removed sheet Y2
- removed sheet Y3
- added sheet S1 (led_group_595.kicad_sch)
- added sheet S10 (led_group_595.kicad_sch)
- added sheet S11 (led_group_595.kicad_sch)
- added sheet S12 (led_group_595.kicad_sch)
- added sheet S13 (led_group_595.kicad_sch)
- added sheet S14 (led_group_595.kicad_sch)
- added sheet S15 (led_group_595.kicad_sch)
- added sheet S16 (led_group_595.kicad_sch)
- added sheet S17 (led_group_595.kicad_sch)
- added sheet S18 (led_group_595.kicad_sch)
- added sheet S19 (led_group_595.kicad_sch)
- added sheet S2 (led_group_595.kicad_sch)
- added sheet S20 (led_group_595.kicad_sch)
- added sheet S21 (led_group_595.kicad_sch)
- added sheet S22 (led_group_595.kicad_sch)
- added sheet S23 (led_group_595.kicad_sch)
- added sheet S24 (led_group_595.kicad_sch)
- added sheet S3 (led_group_595.kicad_sch)
- added sheet S4 (led_group_595.kicad_sch)
- added sheet S5 (led_group_595.kicad_sch)
- added sheet S6 (led_group_595.kicad_sch)
- added sheet S7 (led_group_595.kicad_sch)
- added sheet S8 (led_group_595.kicad_sch)
- added sheet S9 (led_group_595.kicad_sch)
- moved on the sheet: C1, C2, C3, C4, C5, C6, D_DOOR_G1, D_DOOR_Y1, D_ISL_ADM1, D_ISL_ADM_CEN1, D_ISL_ADM_WAC1, D_ISL_CAB_TIH1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

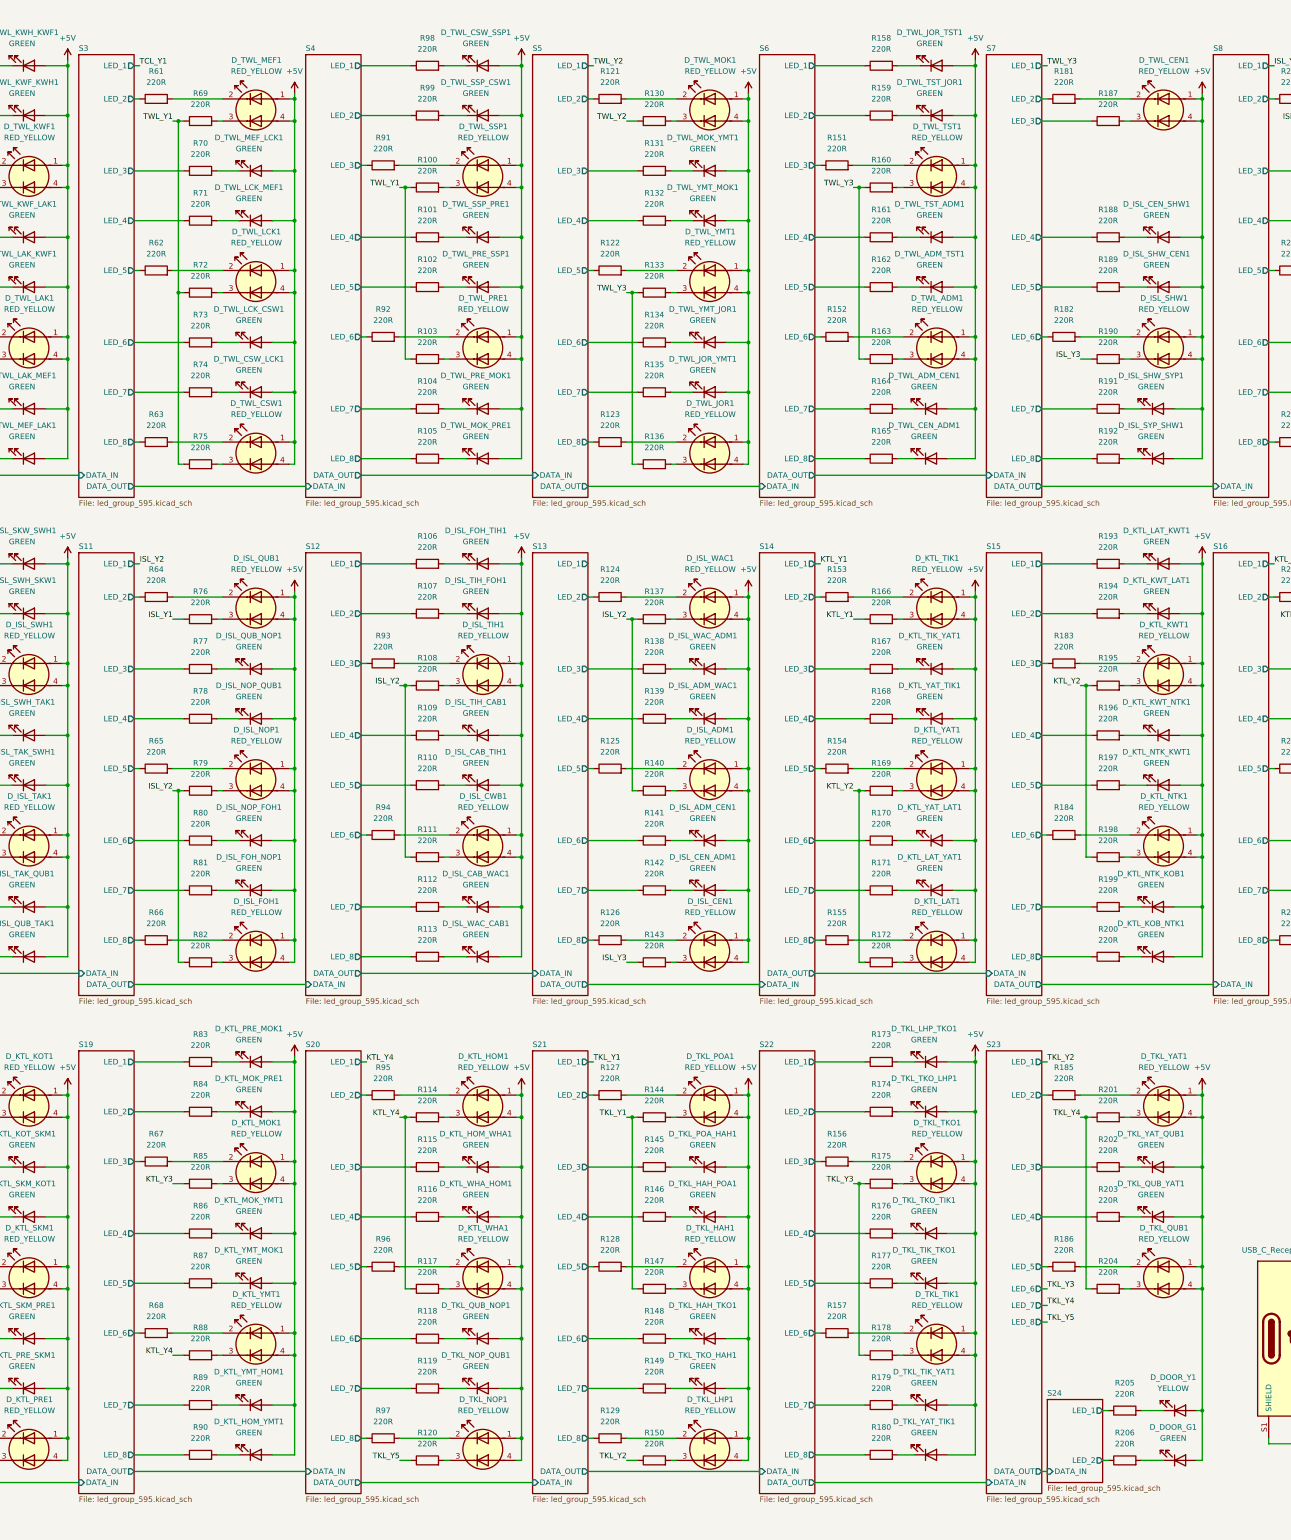
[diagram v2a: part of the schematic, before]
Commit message: PCB track routing part 3
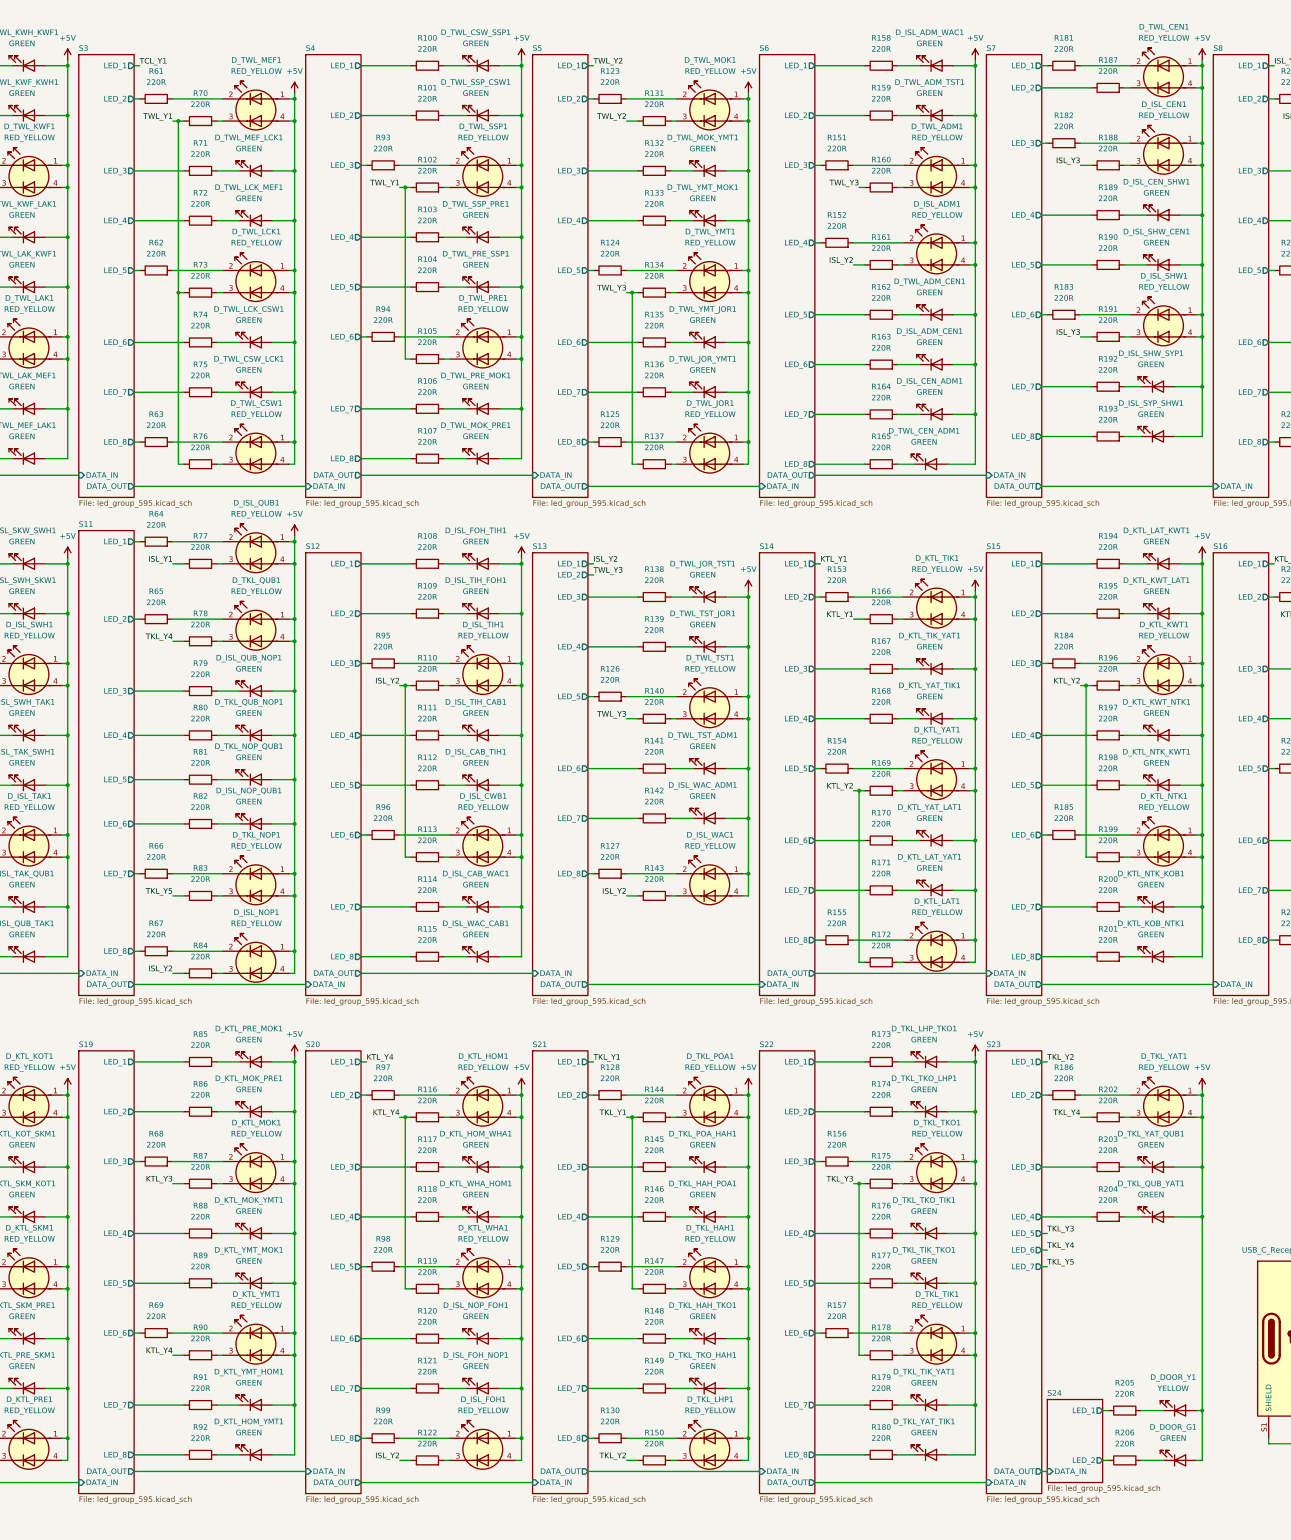
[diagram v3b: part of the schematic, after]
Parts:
- renumbered R98 to R100, R99 to R101, R100 to R102, R101 to R103, R102 to R104, R103 to R105, R104 to R106, R105 to R107, R106 to R108, R107 to R109, R108 to R110, R109 to R111, R110 to R112, R111 to R113, R112 to R114, R113 to R115, R114 to R116, R115 to R117, R116 to R118, R117 to R119, R80 to R120, R81 to R121, R82 to R122, R121 to R123, R122 to R124, R123 to R125, R151 to R126, R124 to R127, R127 to R128, R128 to R129, R129 to R130, R130 to R131, R131 to R132, R132 to R133, R133 to R134, R134 to R135, R135 to R136, R136 to R137, R158 to R138, R159 to R139, R160 to R140, R161 to R141, R138 to R142, R137 to R143, R152 to R151, R125 to R152, R139 to R158, R162 to R159, R163 to R160, R140 to R161, R164 to R162, R141 to R163, R142 to R164, R126 to R182, R182 to R183, R183 to R184, R184 to R185, R185 to R186, R143 to R188, R188 to R189, R189 to R190, R190 to R191, R191 to R192, R192 to R193, R193 to R194, R194 to R195, R195 to R196, R196 to R197, R197 to R198, R198 to R199, R199 to R200, R200 to R201, R201 to R202, R202 to R203, R203 to R204, R186 to R65, R97 to R66, R65 to R67, R67 to R68, R68 to R69, R69 to R70, R70 to R71, R71 to R72, R72 to R73, R73 to R74, R74 to R75, R75 to R76, R76 to R77, R204 to R78, R77 to R79, R118 to R80, R119 to R81, R78 to R82, R120 to R83, R79 to R84, R83 to R85, R84 to R86, R85 to R87, R86 to R88, R87 to R89, R88 to R90, R89 to R91, R90 to R92, R91 to R93, R92 to R94, R93 to R95, R94 to R96, R95 to R97, R96 to R98, R66 to R99
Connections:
- net S13/LED_2 is gone; now on net S13/LED_8: R127.1
- net S23/LED_5 is gone; now on net S11/LED_2: R65.1
- net S11/LED_2: no longer R64.1
- net S11/LED_4: now also R80.1; no longer R82.1
- net S11/LED_5: now also R81.1; no longer R67.1
- net S11/LED_6: now also R82.1; no longer R120.1
- net S11/LED_7: now also R66.1; no longer R121.1
- net S11/LED_8: now also R67.1; no longer R99.1
- net S13/LED_3: now also R138.1; no longer R142.1
- net S13/LED_4: now also R139.1; no longer R158.1
- net S13/LED_5: now also R126.1; no longer R152.1
- net S13/LED_6: now also R141.1; no longer R163.1
- net S13/LED_7: now also R142.1; no longer R164.1
- net S13/LED_8: no longer R182.1
- net S20/LED_6: now also R120.1; no longer R80.1
- net S20/LED_7: now also R121.1; no longer R81.1
- net S20/LED_8: now also R99.1; no longer R66.1
- net S6/LED_1: now also R158.1; no longer R138.1
- net S6/LED_2: now also R159.1; no longer R139.1
- net S6/LED_3: now also R151.1; no longer R126.1
- net S6/LED_4: now also R152.1; no longer R141.1
- net S6/LED_5: now also R162.1; no longer R159.1
- net S6/LED_6: now also R163.1; no longer R151.1
- net S6/LED_7: now also R164.1; no longer R162.1
- net S7/LED_2: now also R187.1; no longer R181.1
- net S7/LED_3: now also R182.1; no longer R187.1
- new net S11/LED_1: R64.1
- new net S7/LED_1: R181.1
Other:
- sheet S23 ports: added none; removed LED_8
- moved on the sheet: D_ISL_ADM1, D_ISL_ADM_CEN1, D_ISL_ADM_WAC1, D_ISL_CEN1, D_ISL_CEN_ADM1, D_ISL_CEN_SHW1, D_ISL_FOH1, D_ISL_FOH_NOP1, D_ISL_NOP1, D_ISL_NOP_FOH1, D_ISL_NOP_QUB1, D_ISL_QUB1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
